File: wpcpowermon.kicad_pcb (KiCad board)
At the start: 2 copper layers, 75.2 x 66.5 mm, 20 parts, among them J1 Screw_Terminal_01x04, J1001 Conn_02x17_Odd_Even, J2 LED, J3 LED, J4 Screw_Terminal_01x02, U3 74HC245, U4 74HC245, U5 Pico, U6 MAX485E

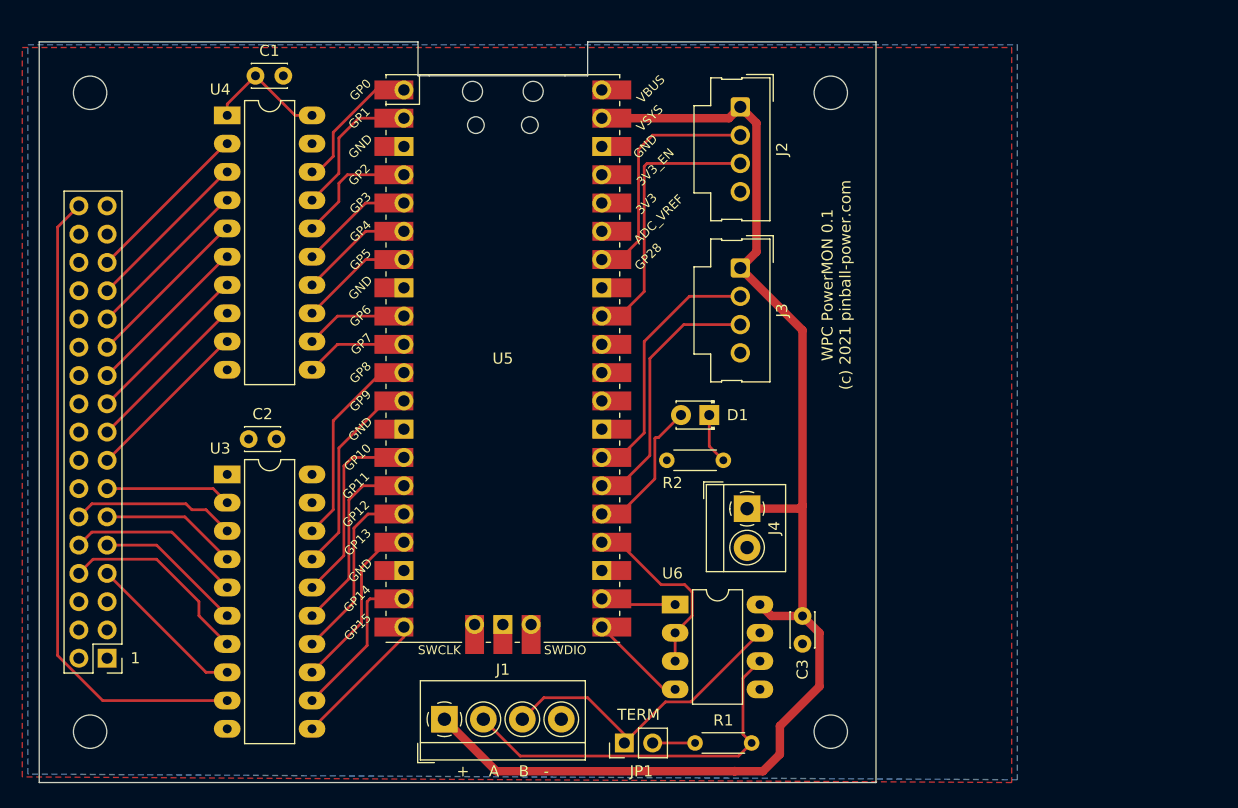
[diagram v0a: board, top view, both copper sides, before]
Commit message: v 0.2
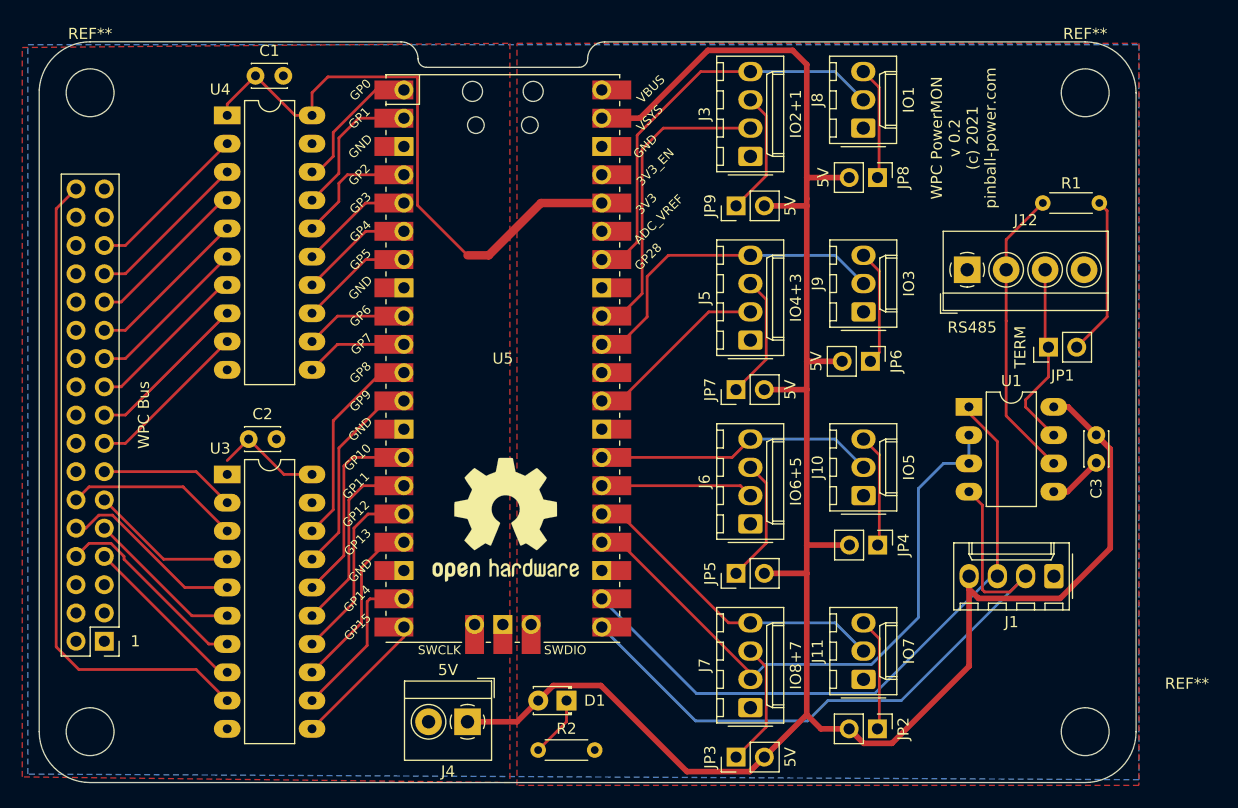
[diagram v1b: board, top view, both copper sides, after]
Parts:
- removed ? (x4): MountingHole_3mm, MountingHole:MountingHole_3mm
- removed J2: LED, Connector_Molex:Molex_SL_171971-0004_1x04_P2.54mm_Vertical
- removed U6: MAX485E, Package_DIP:DIP-8_W7.62mm_LongPads
- added J10: IO5, Connector_Molex:Molex_KK-254_AE-6410-03A_1x03_P2.54mm_Vertical, F.Cu at (154.3, 102.2)
- added J11: IO7, Connector_Molex:Molex_KK-254_AE-6410-03A_1x03_P2.54mm_Vertical, F.Cu at (154.3, 118.7)
- added J12: RS485, TerminalBlock_4Ucon:TerminalBlock_4Ucon_1x04_P3.50mm_Horizontal, F.Cu at (163.6, 81.9)
- added J5: IO4+3, Connector_Molex:Molex_KK-254_AE-6410-04A_1x04_P2.54mm_Vertical, F.Cu at (144.2, 88.3)
- added J6: IO6+5, Connector_Molex:Molex_KK-254_AE-6410-04A_1x04_P2.54mm_Vertical, F.Cu at (144.2, 104.8)
- added J7: IO8+7, Connector_Molex:Molex_KK-254_AE-6410-04A_1x04_P2.54mm_Vertical, F.Cu at (144.2, 121.3)
- added J8: IO1, Connector_Molex:Molex_KK-254_AE-6410-03A_1x03_P2.54mm_Vertical, F.Cu at (154.3, 69.2)
- added J9: IO3, Connector_Molex:Molex_KK-254_AE-6410-03A_1x03_P2.54mm_Vertical, F.Cu at (154.3, 85.7)
- added JP2: 5V, Connector_PinHeader_2.54mm:PinHeader_1x02_P2.54mm_Vertical, F.Cu at (155.6, 123.2)
- added JP3: 5V, Connector_PinHeader_2.54mm:PinHeader_1x02_P2.54mm_Vertical, F.Cu at (142.9, 125.7)
- added JP4: 5V, Connector_PinHeader_2.54mm:PinHeader_1x02_P2.54mm_Vertical, F.Cu at (155.6, 106.7)
- added JP5: 5V, Connector_PinHeader_2.54mm:PinHeader_1x02_P2.54mm_Vertical, F.Cu at (142.9, 109.2)
- added JP6: 5V, Connector_PinHeader_2.54mm:PinHeader_1x02_P2.54mm_Vertical, F.Cu at (154.9, 90.2)
- added JP7: 5V, Connector_PinHeader_2.54mm:PinHeader_1x02_P2.54mm_Vertical, F.Cu at (142.9, 92.7)
- added JP8: 5V, Connector_PinHeader_2.54mm:PinHeader_1x02_P2.54mm_Vertical, F.Cu at (155.6, 73.7)
- added JP9: 5V, Connector_PinHeader_2.54mm:PinHeader_1x02_P2.54mm_Vertical, F.Cu at (142.9, 76.2)
- added REF**: MountingHole_4.3mm_M4, MountingHole:MountingHole_4.3mm_M4, F.Cu at (84.8, 66.0)
- added REF**: MountingHole_4.3mm_M4, MountingHole:MountingHole_4.3mm_M4, F.Cu at (174.2, 66.0)
- added REF**: MountingHole_4.3mm_M4, MountingHole:MountingHole_4.3mm_M4, F.Cu at (174.2, 123.4)
- added REF**: MountingHole_4.3mm_M4, MountingHole:MountingHole_4.3mm_M4, F.Cu at (84.8, 123.4)
- added REF**: OSHW-Logo2_14.6x12mm_SilkScreen, Symbol:OSHW-Logo2_14.6x12mm_SilkScreen, F.Cu at (122.2, 104.4)
- added U1: MAX485E, Package_DIP:DIP-8_W7.62mm_LongPads, F.Cu at (163.8, 94.3)
- J1: value Screw_Terminal_01x04 -> RS232; footprint TerminalBlock_4Ucon:TerminalBlock_4Ucon_1x04_P3.50mm_Horizontal -> Connector_Molex:Molex_KK-254_AE-6410-04A_1x04_P2.54mm_Vertical
- J1001: value Conn_02x17_Odd_Even -> WPC Bus
- J3: value LED -> IO2+1; footprint Connector_Molex:Molex_SL_171971-0004_1x04_P2.54mm_Vertical -> Connector_Molex:Molex_KK-254_AE-6410-04A_1x04_P2.54mm_Vertical
- J4: value Screw_Terminal_01x02 -> 5V
- JP1: value Jumper -> TERM
- moved J1 56.2 mm to (171.4, 109.5), turned to 180 degrees
- moved R1 55.1 mm to (170.4, 75.9), turned to 0 degrees
- moved JP1 52.1 mm to (170.9, 88.9)
- moved J4 31.6 mm to (118.7, 122.6), turned to 180 degrees
- moved C3 31.0 mm to (175.2, 96.8)
- moved R2 30.9 mm to (125.1, 125.1), turned to 0 degrees
- moved D1 28.7 mm to (127.6, 120.7)
- moved J3 10.1 mm to (144.2, 71.8), turned to 90 degrees
- moved J1001 1.55 mm to (86.1, 115.3)
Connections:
- D1 pad 2: Net-(D1-Pad2) -> +5V
- J1 pad 1: +5V -> GND
- J1 pad 2: Net-(R1-Pad1) -> /io/TX
- J1 pad 3: Net-(JP1-Pad1) -> /io/RX
- J1 pad 4: GND -> +5V
- J3 pad 1: +5V -> GND
- J3 pad 2: Net-(J3-Pad2) -> /io/IO2
- J3 pad 4: GND -> /io/IO1
- JP1 pad 1: Net-(JP1-Pad1) -> Net-(J12-Pad3)
- R1 pad 1: Net-(R1-Pad1) -> Net-(J12-Pad2)
- U5 pad 21: Net-(U5-Pad21) -> /io/TX
- U5 pad 22: Net-(U5-Pad22) -> /io/RX
- U5 pad 24: Net-(U5-Pad24) -> /io/IO8
- U5 pad 25: Net-(D1-Pad2) -> /io/IO7
- U5 pad 26: Net-(J3-Pad3) -> /io/IO6
- U5 pad 27: Net-(J3-Pad2) -> /io/IO5
- U5 pad 29: unconnected-(U5-Pad29) -> /io/IO4
- U5 pad 31: unconnected-(U5-Pad31) -> /io/IO3
- U5 pad 32: Net-(J2-Pad3) -> /io/IO2
- U5 pad 34: Net-(J2-Pad2) -> /io/IO1
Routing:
- net +5V: track 118.7 -> 197.6 mm
- net /io/TX: track 0.00 -> 60.8 mm
- net /io/RX: track 0.00 -> 59.7 mm
- net /io/IO8: track 0.00 -> 55.8 mm
- net +3V3: track 11.2 -> 64.9 mm
- net /io/IO1: track 0.00 -> 37.2 mm
- net Net-(R1-Pad1): track 34.3 -> 0.00 mm
- net /io/IO3: track 0.00 -> 30.0 mm
- net /io/IO7: track 0.00 -> 28.6 mm
- net Net-(JP1-Pad1): track 28.4 -> 0.00 mm
- net /io/IO2: track 0.00 -> 27.9 mm
- net Net-(J12-Pad2): track 0.00 -> 26.5 mm
- net /io/IO5: track 0.00 -> 25.3 mm
- net Net-(J2-Pad3): track 23.1 -> 0.00 mm
- net Net-(J3-Pad2): track 21.6 -> 0.00 mm
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- added copper zone on F.Cu, net +5V
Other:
- board size 75.2 x 66.5 mm -> 98.6 x 66.6 mm
- board text added: "WPC PowerMON v 0.2 (c) 2021 pinball-power.com"
- board text removed: "+ A B -"
- board text removed: "TERM"
- board text removed: "WPC PowerMON 0.1 (c) 2021 pinball-power.com"
